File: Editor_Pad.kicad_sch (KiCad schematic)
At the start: 1 part

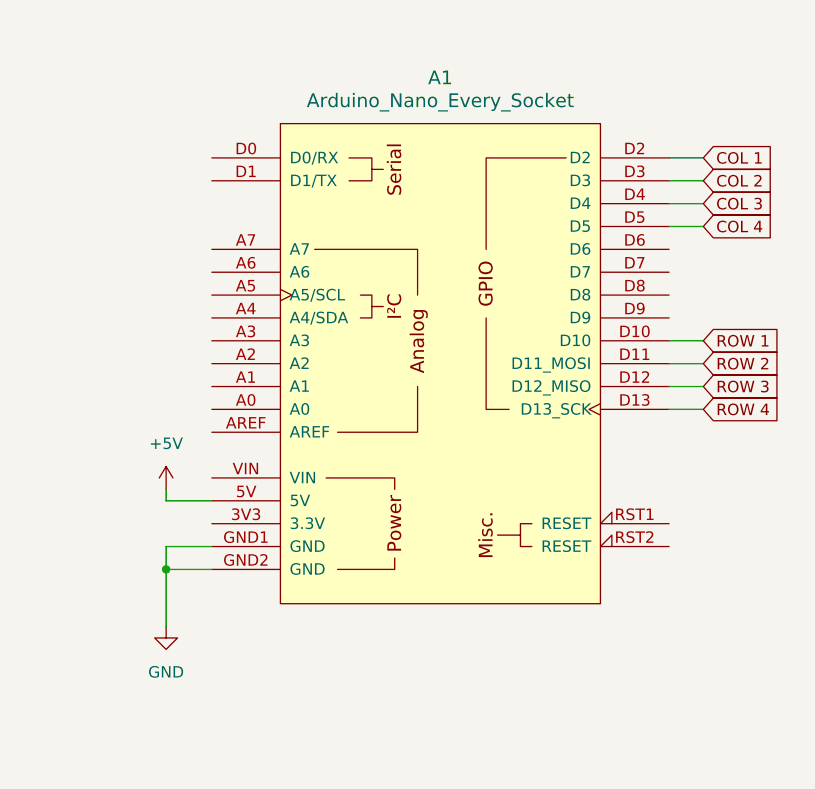
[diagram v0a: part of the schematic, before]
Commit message: Working on a proper routing
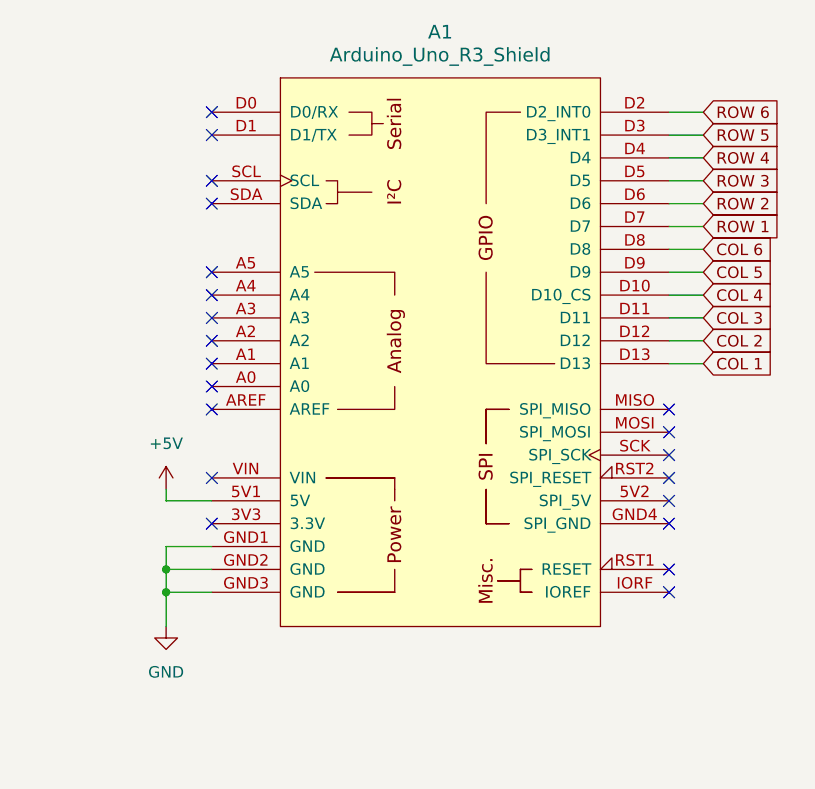
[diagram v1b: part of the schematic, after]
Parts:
- removed A1: Arduino_Nano_Every_Socket, PCM_arduino-library:Arduino_Nano_Every_Socket, symbol PCM_arduino-library:Arduino_Nano_Every_Socket
- added A1: Arduino_Uno_R3_Shield, PCM_arduino-library:Arduino_Uno_R3_Shield, symbol PCM_arduino-library:Arduino_Uno_R3_Shield
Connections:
- net +5V: now also A1.5V1 (5V)
- net COL 1: now also A1.D13
- net COL 2: now also A1.D12
- net COL 3: now also A1.D11
- net COL 4: now also A1.D10 (D10_CS)
- net GND: now also A1.GND1 (GND), A1.GND2 (GND), A1.GND3 (GND)
- net ROW 1: now also A1.D7
- net ROW 2: now also A1.D6
- net ROW 3: now also A1.D5
- net ROW 4: now also A1.D4
- new net COL 5: A1.D9
- new net COL 6: A1.D8
- new net ROW 5: A1.D3 (D3_INT1)
- new net ROW 6: A1.D2 (D2_INT0)
- no-connect marks 0 -> 21

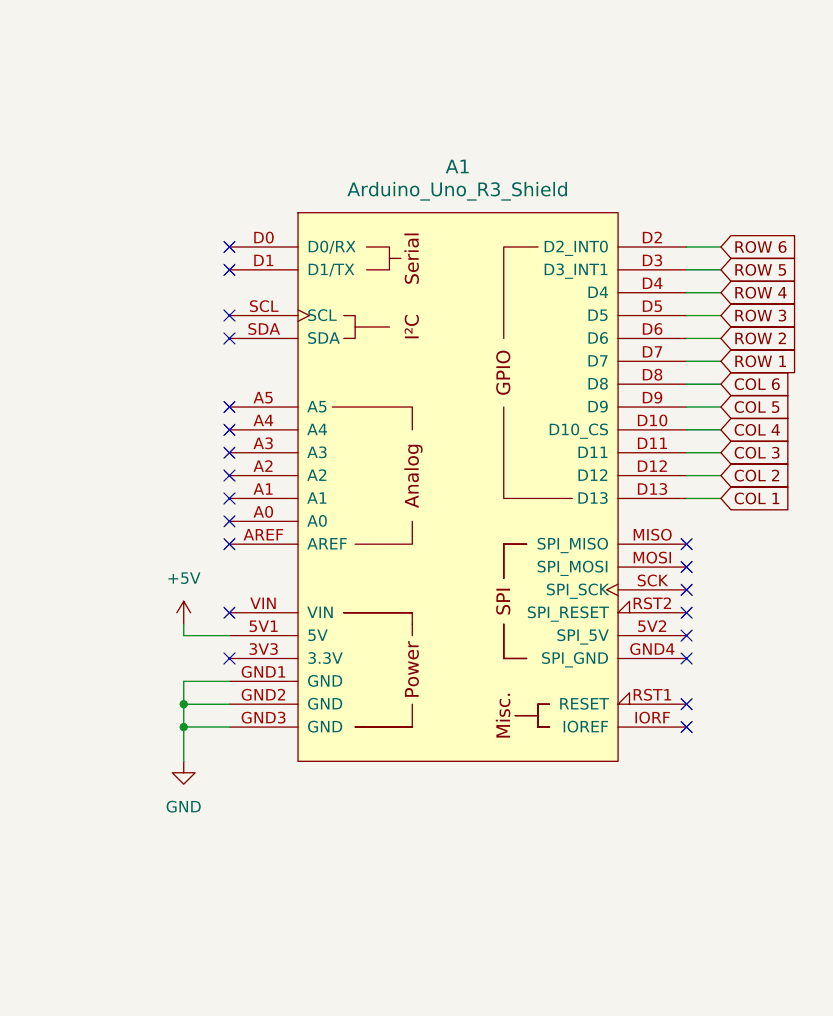
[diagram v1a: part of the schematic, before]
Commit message: Slightly modified
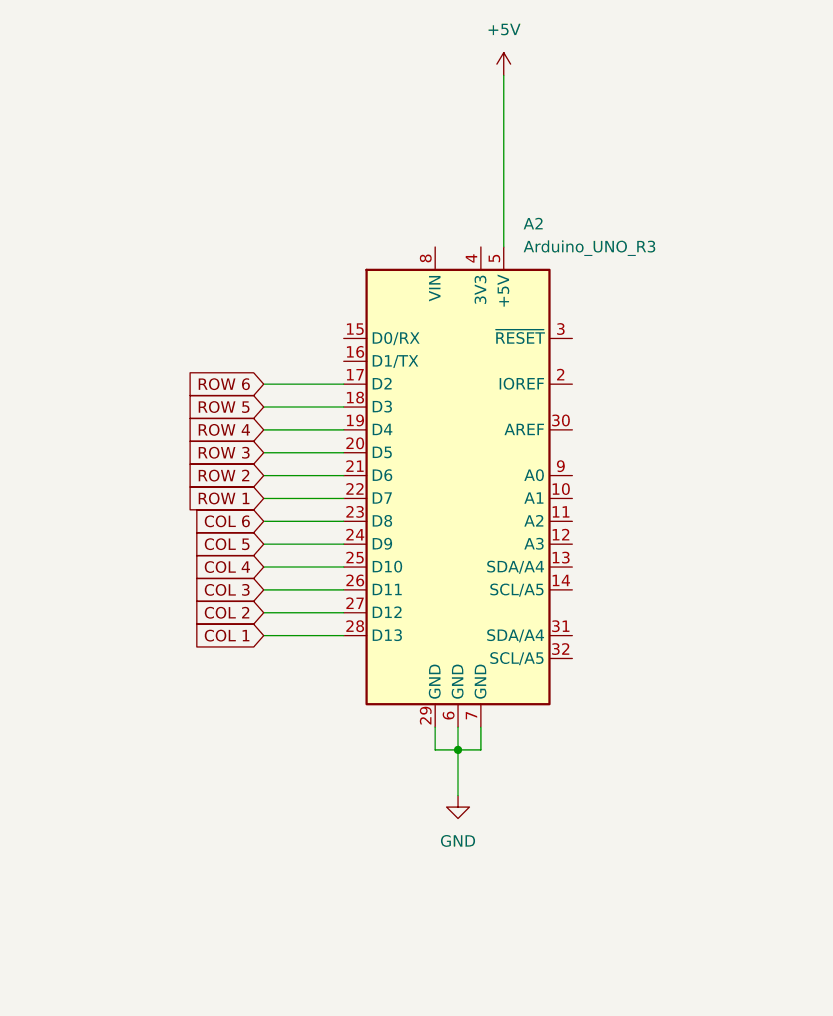
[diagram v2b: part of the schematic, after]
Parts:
- removed A1: Arduino_Uno_R3_Shield, PCM_arduino-library:Arduino_Uno_R3_Shield, symbol PCM_arduino-library:Arduino_Uno_R3_Shield
- added A2: Arduino_UNO_R3, Module:Arduino_UNO_R3, symbol MCU_Module:Arduino_UNO_R3
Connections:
- net +5V: now also A2.5 (+5V)
- net COL 1: now also A2.28 (D13)
- net COL 2: now also A2.27 (D12)
- net COL 3: now also A2.26 (D11)
- net COL 4: now also A2.25 (D10)
- net COL 5: now also A2.24 (D9)
- net COL 6: now also A2.23 (D8)
- net GND: now also A2.29 (GND), A2.6 (GND), A2.7 (GND)
- net ROW 1: now also A2.22 (D7)
- net ROW 2: now also A2.21 (D6)
- net ROW 3: now also A2.20 (D5)
- net ROW 4: now also A2.19 (D4)
- net ROW 5: now also A2.18 (D3)
- net ROW 6: now also A2.17 (D2)
- no-connect marks 21 -> 0
